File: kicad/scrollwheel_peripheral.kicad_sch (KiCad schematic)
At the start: 24 parts, among them IC1 ATMEGA32U4-AU, J1 UJ20-C-H-G-MSMT-4-P16-TR, J2 AVR-JTAG-10, J3 TSW-110-07-F-D, SW1 SW_Push_Dual, Y1 Crystal

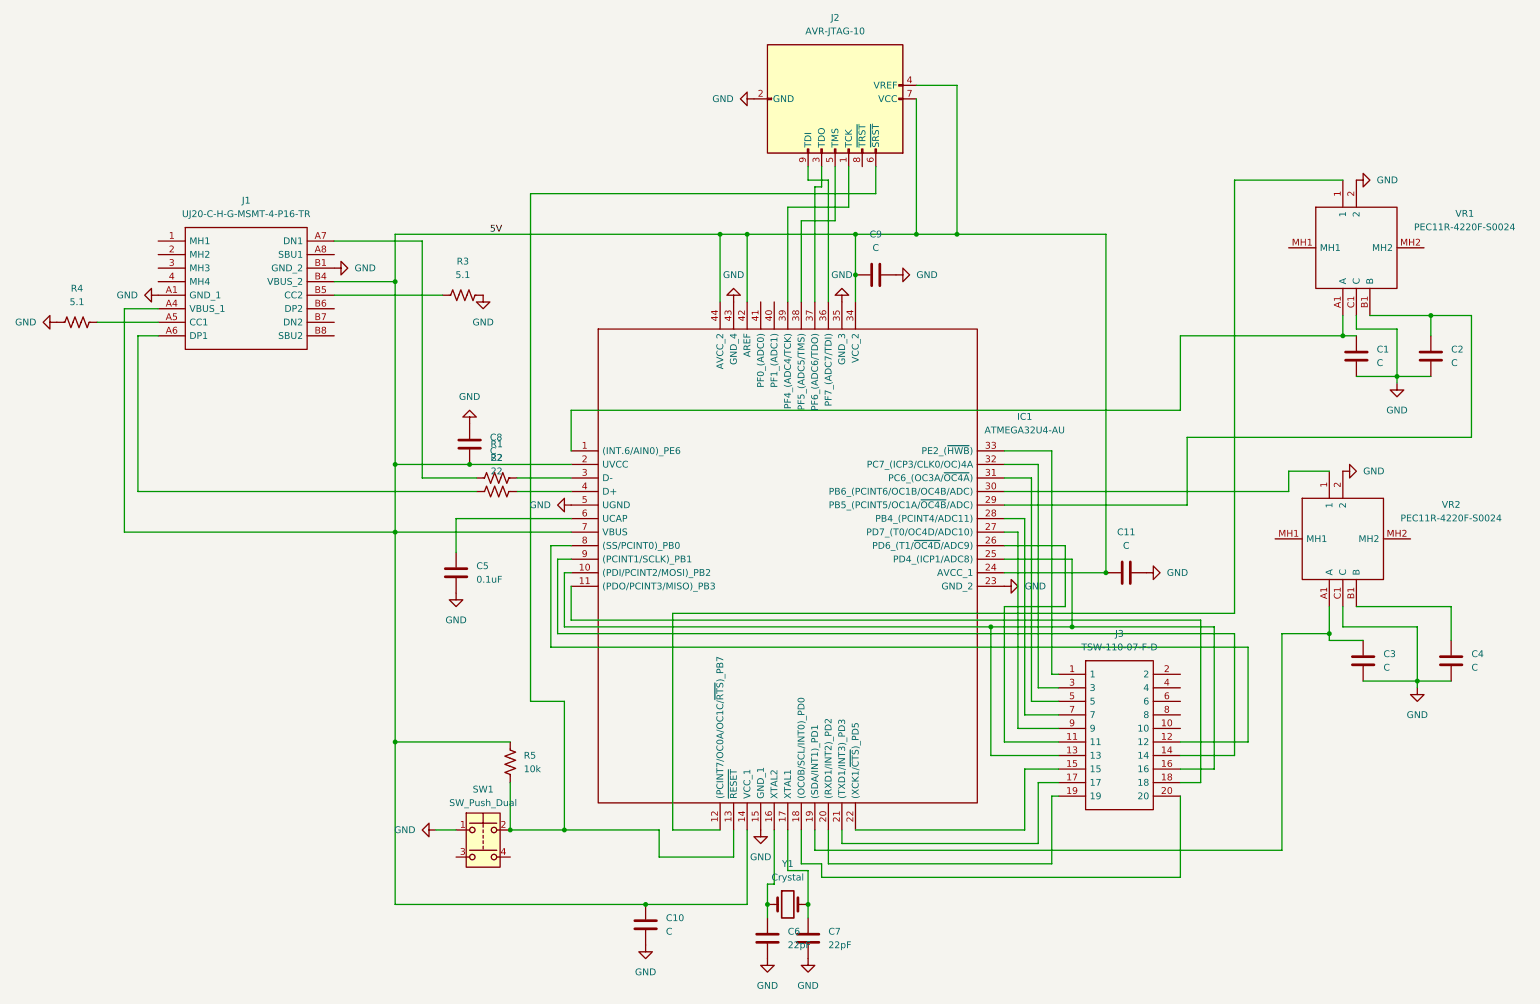
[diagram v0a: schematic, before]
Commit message: Finish routing for rev 1
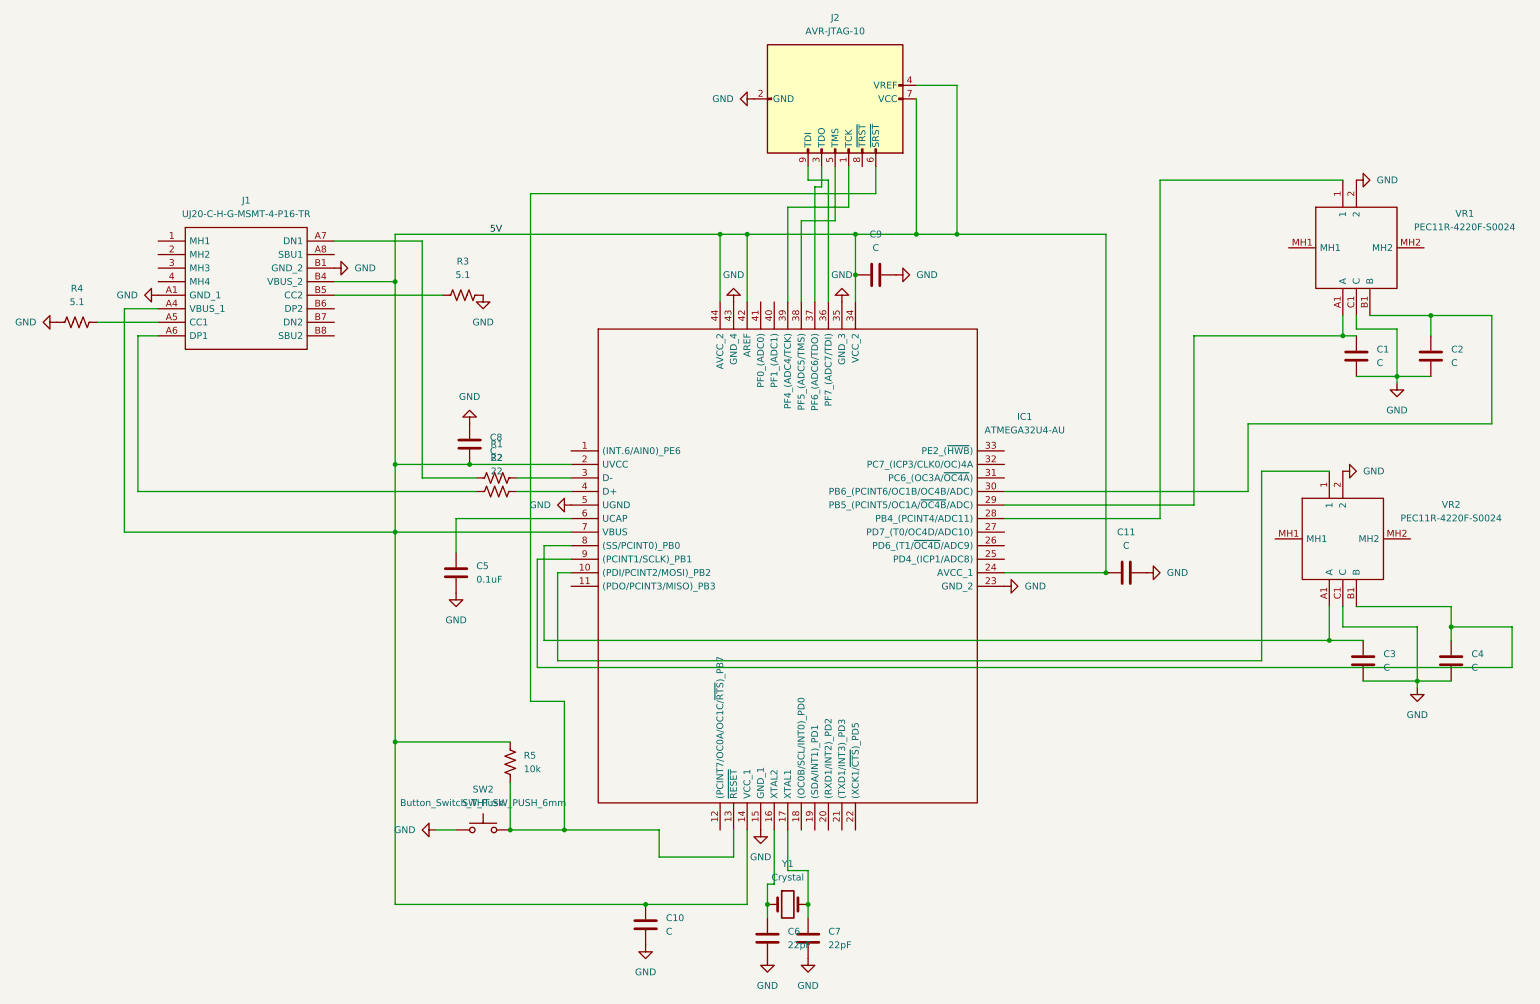
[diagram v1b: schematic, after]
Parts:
- removed J3: TSW-110-07-F-D, project_footprints:TSW-110-XX-YY-D, symbol TSW-110-07-F-D:TSW-110-07-F-D
- removed SW1: SW_Push_Dual, Button_Switch_THT:SW_PUSH_6mm, symbol Switch:SW_Push_Dual
- added SW2: SW_Push, Button_Switch_THT:SW_PUSH_6mm, symbol Switch:SW_Push
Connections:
- net GND: now also SW2.1
- net at C2.1, VR1.B1 (B): now also IC1.30 (PB6_(PCINT6/OC1B/OC4B/ADC)); no longer IC1.29 (PB5_(PCINT5/OC1A/~{OC4B}/ADC))
- net at VR1.1: now also IC1.28 (PB4_(PCINT4/ADC11)); no longer IC1.12 ((PCINT7/OC0A/OC1C/~{RTS})_PB7)
- net at C1.1, VR1.A1 (A): now also IC1.29 (PB5_(PCINT5/OC1A/~{OC4B}/ADC)); no longer IC1.1 ((INT.6/AIN0)_PE6)
- net at VR2.1: now also IC1.10 ((PDI/PCINT2/MOSI)_PB2); no longer IC1.30 (PB6_(PCINT6/OC1B/OC4B/ADC))
- net at C3.1, VR2.A1 (A): now also IC1.8 ((SS/PCINT0)_PB0); no longer IC1.19 ((SDA/INT1)_PD1)
- net at C4.1, VR2.B1 (B): now also IC1.9 ((PCINT1/SCLK)_PB1)
- net at IC1.13 (~{RESET}), J2.6 (~{SRST}), R5.2: now also SW2.2
- net at IC1.25 (PD4_(ICP1/ADC8)): no longer IC1.10 ((PDI/PCINT2/MOSI)_PB2)
